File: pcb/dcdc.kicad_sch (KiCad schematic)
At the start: 31 parts, among them IC2 TPS61240DRVT, U3 TPS54360DDA, U4 SY8088AAC

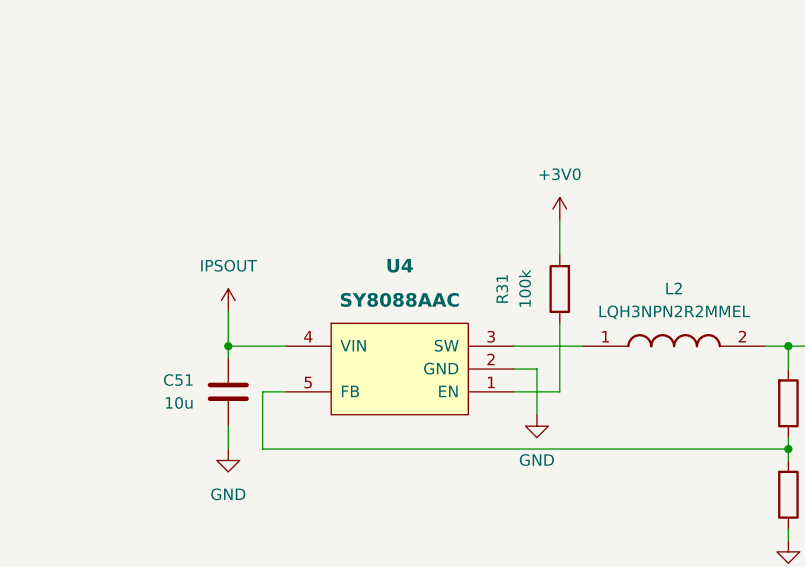
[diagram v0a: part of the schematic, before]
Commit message: Cleaning
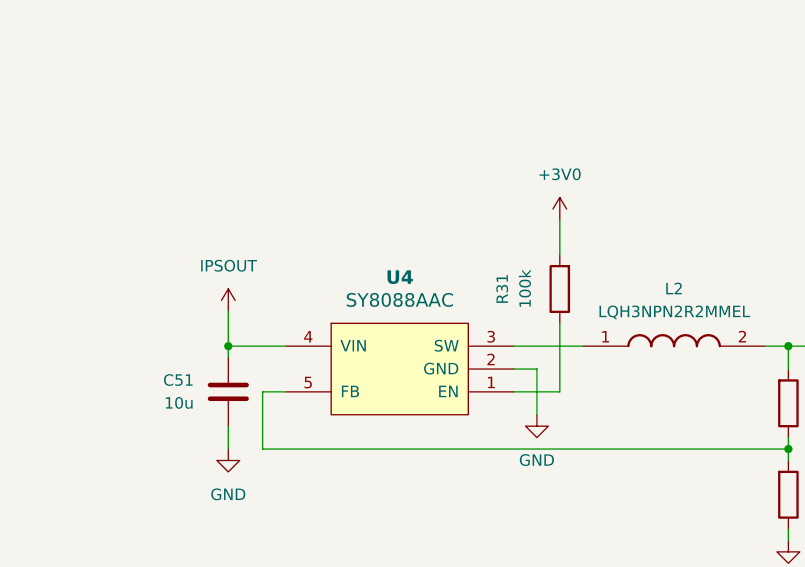
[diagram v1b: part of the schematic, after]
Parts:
- U4: footprint FunKey:SOT23-5 -> Package_TO_SOT_SMD:SOT-23-5
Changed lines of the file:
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@@
 		(fields_autoplaced yes)
 		(property "Reference" "U4"
-			(at 54.61 144.78 0)
+			(at 54.61 146.05 0)
 			(show_name no)
 			(do_not_autoplace no)
@@
 				(font
 					(size 1.4986 1.4986)
-					(bold yes)
+					(thickness 0.1873)
 				)
 			)
 		)
-		(property "Footprint" "FunKey:SOT23-5"
+		(property "Footprint" "Package_TO_SOT_SMD:SOT-23-5"
 			(at 54.61 156.21 0)
 			(hide yes)
@@
 			(at 54.61 156.21 0)
 			(hide yes)
-			(show_name no)
-			(do_not_autoplace no)
-			(effects
-				(font
-					(size 1.27 1.27)
-				)
-			)
-		)
-		(property "PARTNO" ""
-			(at 54.61 156.21 0)
-			(hide yes)
